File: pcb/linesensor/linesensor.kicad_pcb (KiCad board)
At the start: 2 copper layers, 21 x 12 mm, 2 parts, among them J1 Conn_01x03_Socket

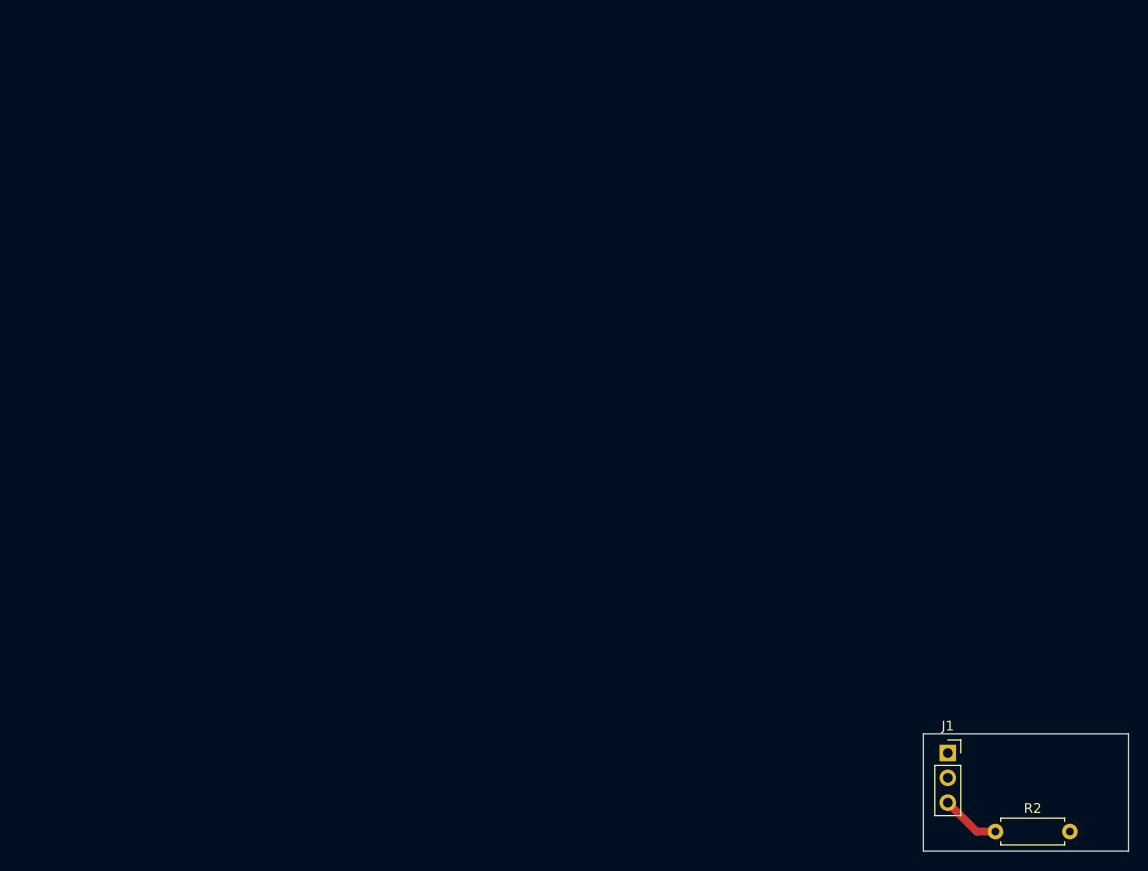
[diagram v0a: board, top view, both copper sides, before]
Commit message: linesensor new
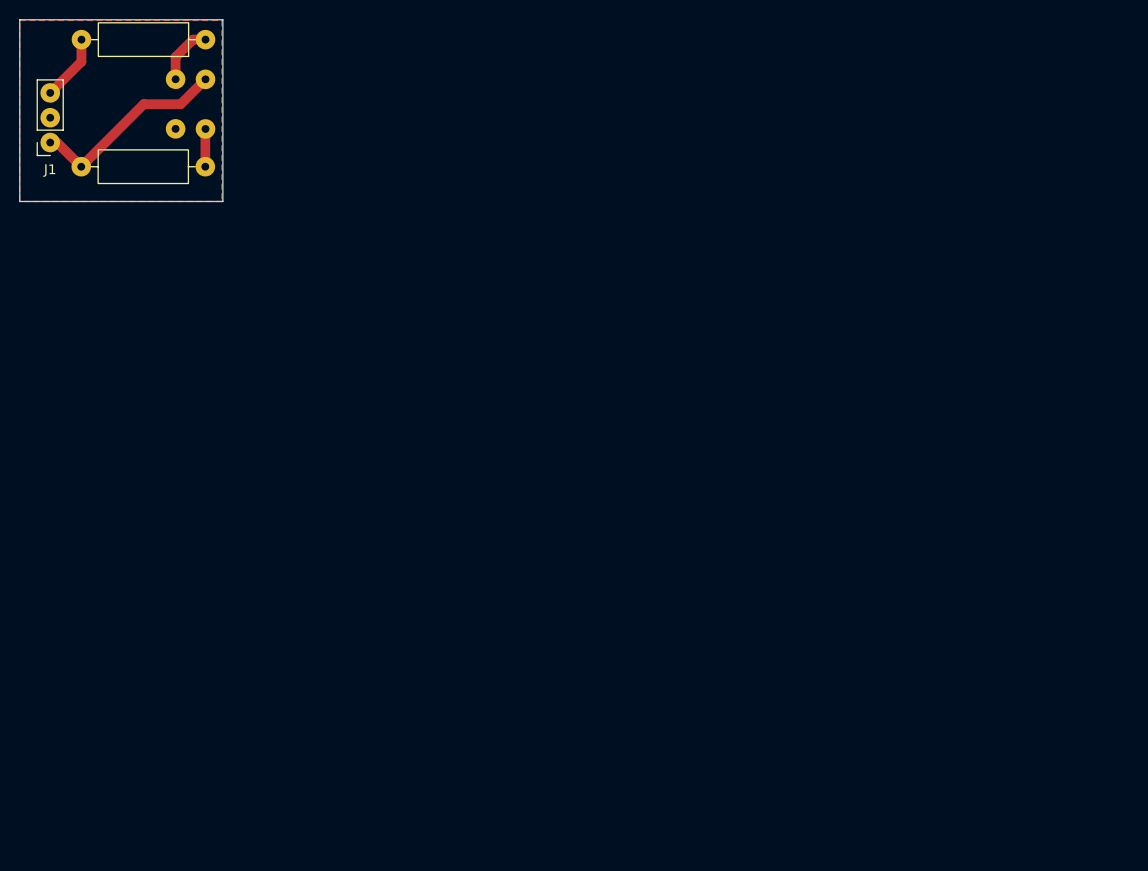
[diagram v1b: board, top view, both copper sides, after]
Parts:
- added R1: R, Resistor_THT:R_Axial_DIN0309_L9.0mm_D3.2mm_P12.70mm_Horizontal, F.Cu at (48.5, 40.4)
- added U1: TRCT5000, Library:CRT5000, F.Cu at (45.5, 34.0)
- R2: value 4,7 -> R; footprint Resistor_THT:R_Axial_DIN0207_L6.3mm_D2.5mm_P7.62mm_Horizontal -> Resistor_THT:R_Axial_DIN0309_L9.0mm_D3.2mm_P12.70mm_Horizontal
- moved R2 114.5 mm to (48.5, 27.4), turned to 180 degrees
- moved J1 111.1 mm to (32.6, 38.0), turned to 180 degrees
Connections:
- J1 pad 2: unconnected-(J1-Pin_2-Pad2) -> GND
- J1 pad 3: GND -> Net-(J1-Pin_3)
- R2 pad 1: GND -> Net-(R2-Pad1)
- R2 pad 2: Net-(R1-Pad2) -> Net-(J1-Pin_3)
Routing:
- net Net-(J1-Pin_1): track 0.00 -> 21.0 mm
- net Net-(J1-Pin_3): track 0.00 -> 6.78 mm
- net GND: track 6.11 -> 0.00 mm
- net Net-(R2-Pad1): track 0.00 -> 6.07 mm
- net Net-(U1A-Vdd): track 0.00 -> 3.47 mm
- added copper zone on F.Cu, net GND
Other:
- board size 21 x 12 mm -> 20.8 x 18.6 mm
